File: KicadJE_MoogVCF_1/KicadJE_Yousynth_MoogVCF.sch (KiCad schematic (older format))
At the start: 99 parts, among them J201 CV2, J202 Input2, J203 CV1, J204 Out VCF, J205 Input1, P201 Doepfer_Power_10pin, Q201 UMX1N, Q202 SS9014, Q203 SS9014, Q204 SS9014, Q205 SS9014, Q206 SS9014, Q207 SS9014, Q208 UMX1N, Q209 UMX1N, Q210 UMX1N, Q211 SS9014, Q212 SS9015, U201 TL072

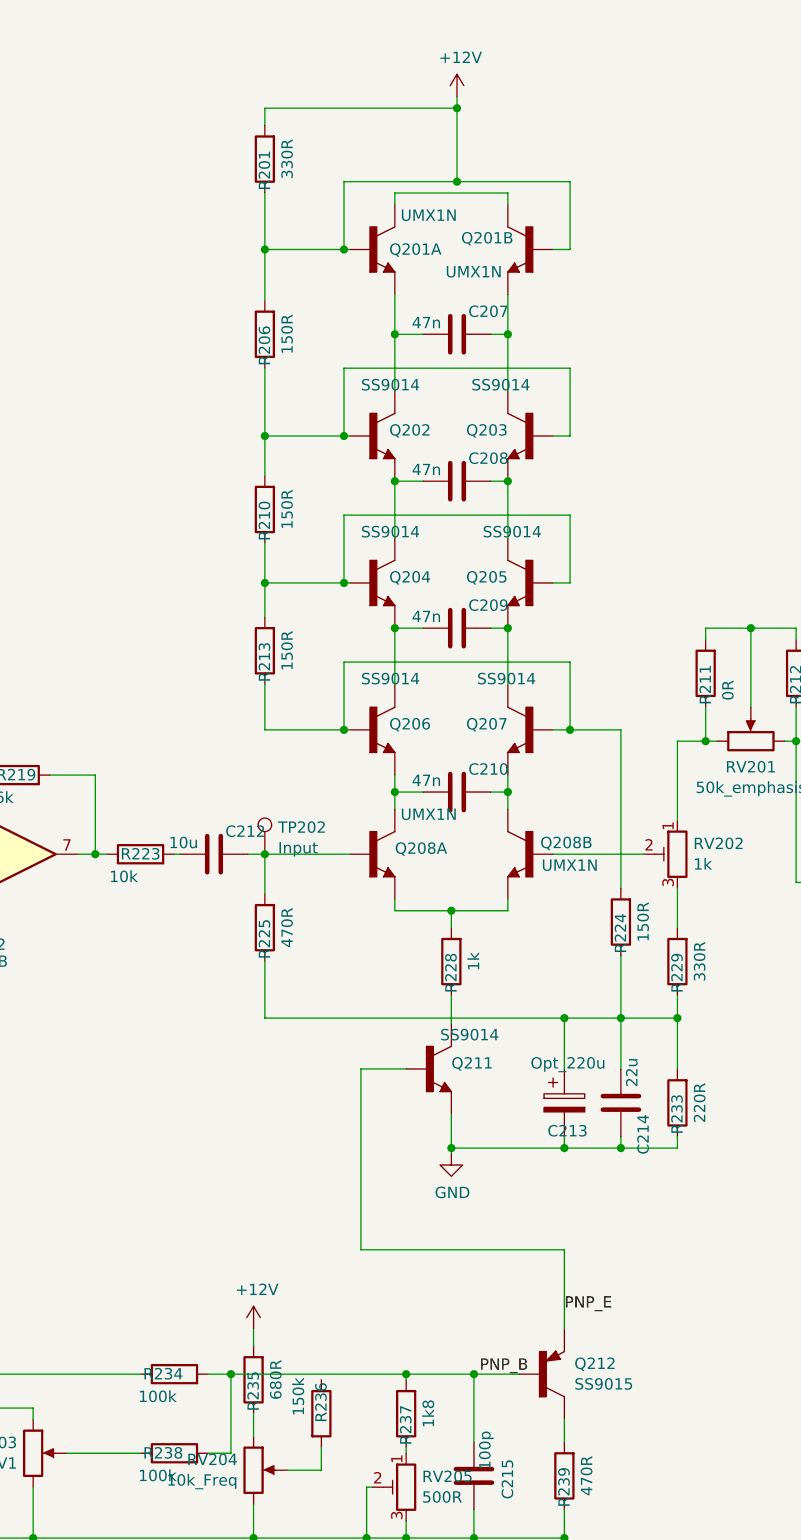
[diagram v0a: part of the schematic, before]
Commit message: all components placed
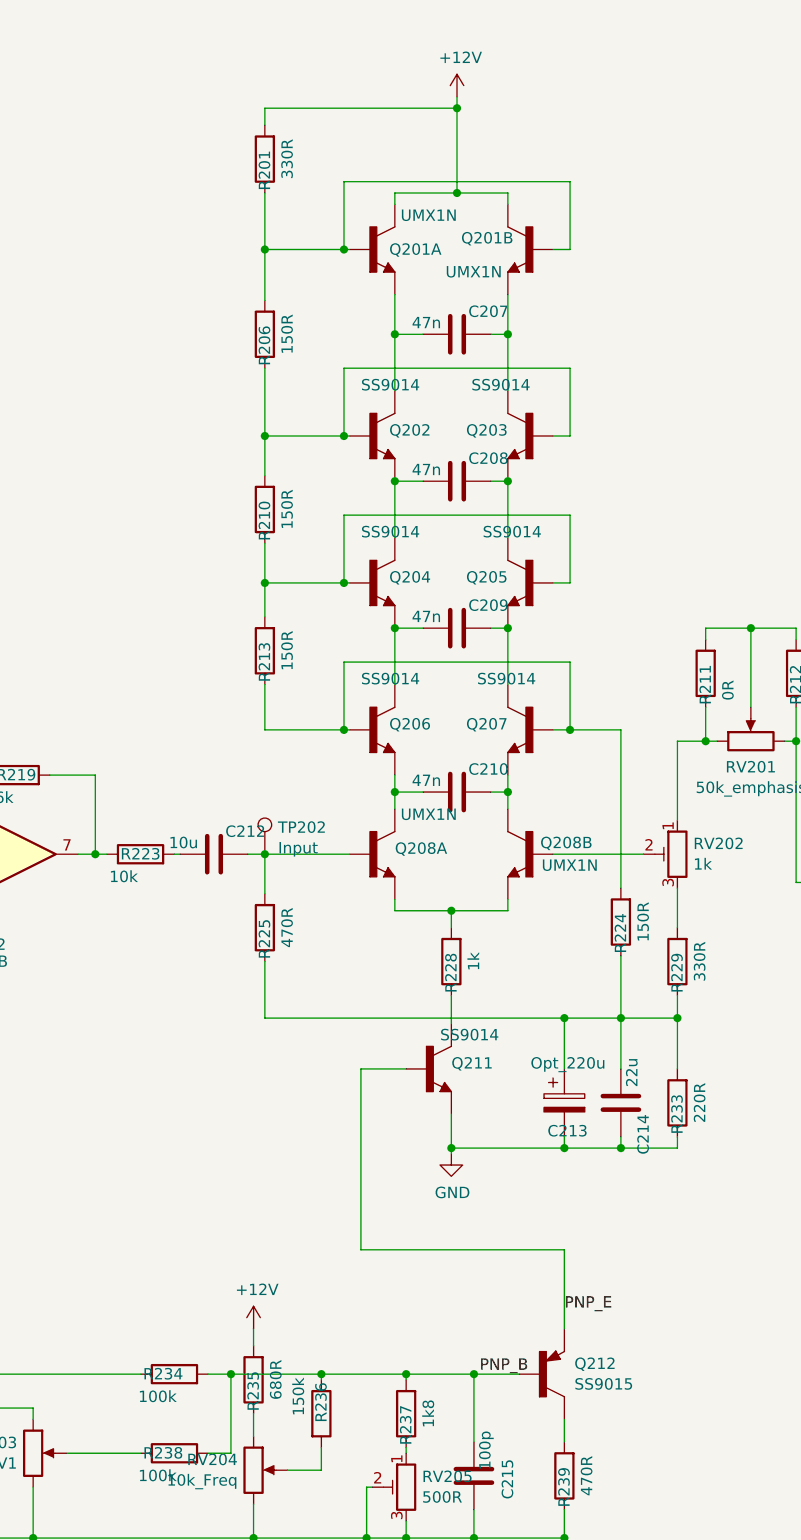
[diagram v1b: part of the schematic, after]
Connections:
- net +12V: now also Q201.3 (C), Q201.6 (C); no longer Q201.2 (B), Q201.5 (B), R201.1, R206.2
- net PNP_B: now also R236.1
- new net: Q201.2 (B), Q201.5 (B), R201.1, R206.2
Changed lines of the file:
@@
 $EndComp
-Wire Wire Line
-	3250 1275 3750 1275
 Wire Wire Line
 	3250 1275 3250 1575
@@
 	3475 1375 3475 1325
 Wire Wire Line
-	3475 1325 3975 1325
+	3475 1325 3750 1325
 Wire Wire Line
 	3975 1325 3975 1375
@@
 	1    0    0    -1
 $EndComp
-Connection ~ 3750 1275
-Wire Wire Line
-	3750 1275 4250 1275
 Wire Wire Line
 	3750 900  3750 950
@@
 Wire Wire Line
 	2900 3700 3250 3700
-Connection ~ 3750 950
-Wire Wire Line
-	3750 950  3750 1275
 Connection ~ 3250 3700
 Wire Wire Line
@@
 Connection ~ 2750 6550
 Wire Wire Line
-	2750 6550 3525 6550
+	2750 6550 3150 6550
 Wire Wire Line
 	3000 6975 3150 6975
@@
 Wire Wire Line
 	7525 1575 7500 1575
+Wire Wire Line
+	3250 1275 4250 1275
+Wire Wire Line
+	3750 950  3750 1325
+Connection ~ 3750 950
+Connection ~ 3750 1325
+Wire Wire Line
+	3750 1325 3975 1325
+Wire Wire Line
+	3150 6575 3150 6550
+Connection ~ 3150 6550
+Wire Wire Line
+	3150 6550 3525 6550
 $EndSCHEMATC
